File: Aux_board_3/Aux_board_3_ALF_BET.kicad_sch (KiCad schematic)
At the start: 37 parts, among them Q10 BSS84KJ, Q11 BSS138KJ, Q12 BSS84KJ, Q13 BSS138KJ, Q14 BSS84KJ, Q15 BSS138KJ, Q16 BSS84KJ, Q7 BSS138KJ, Q8 BSS84KJ, Q9 BSS138KJ

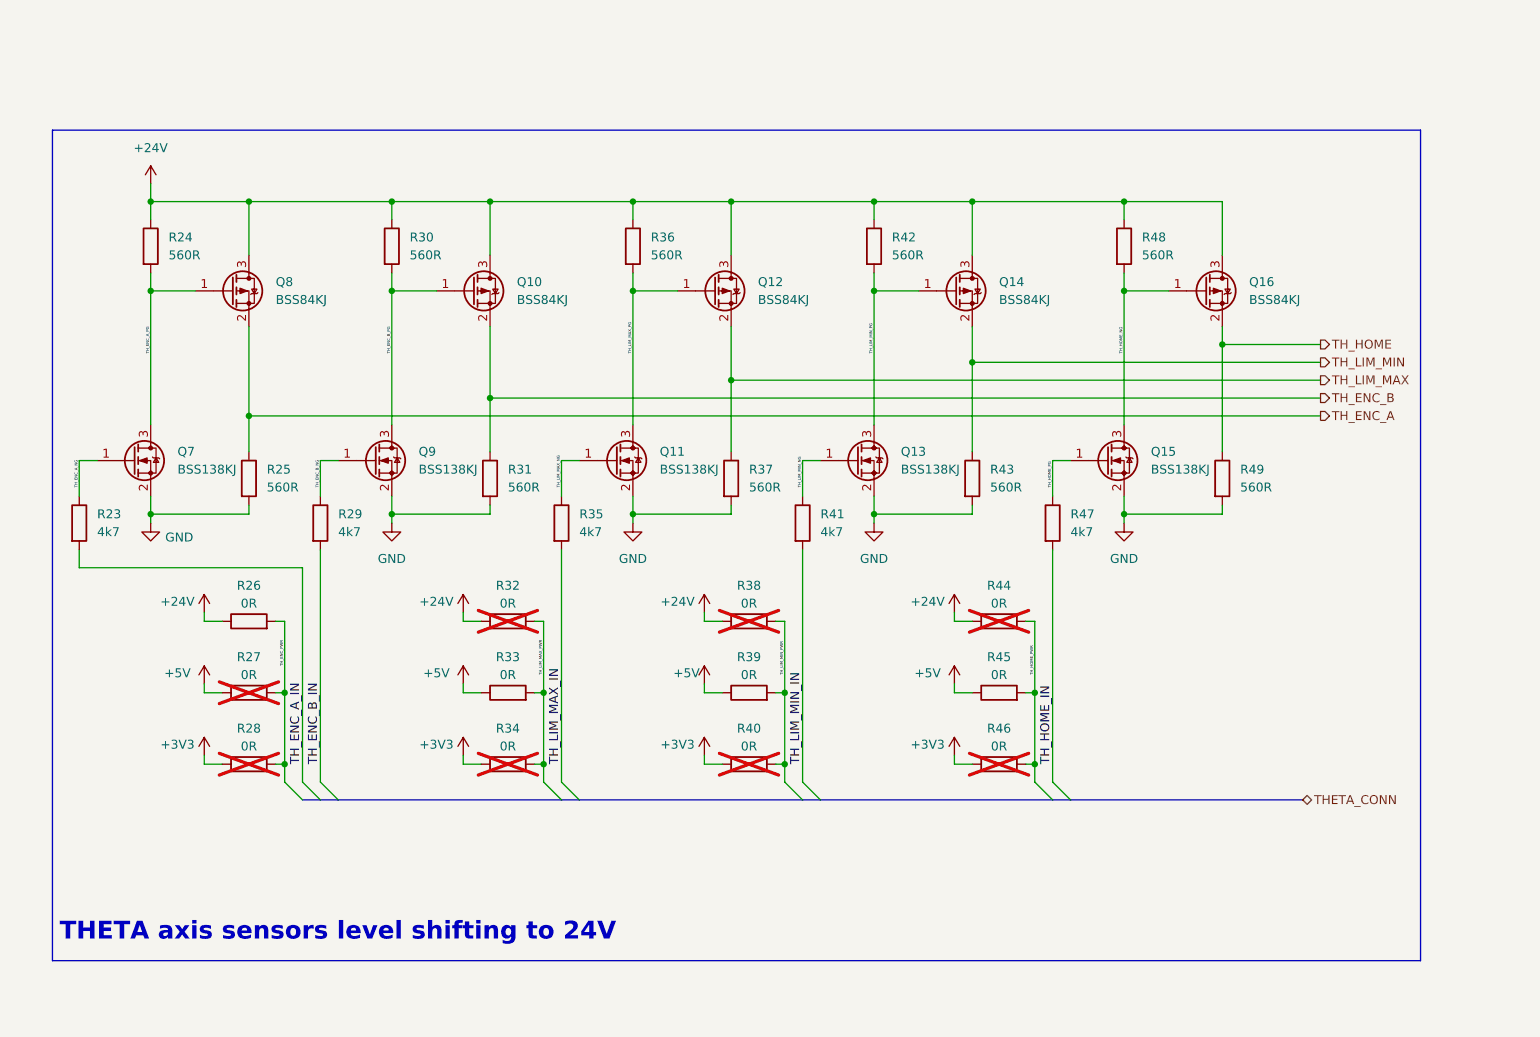
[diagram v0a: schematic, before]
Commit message: finished Board 3 schematic
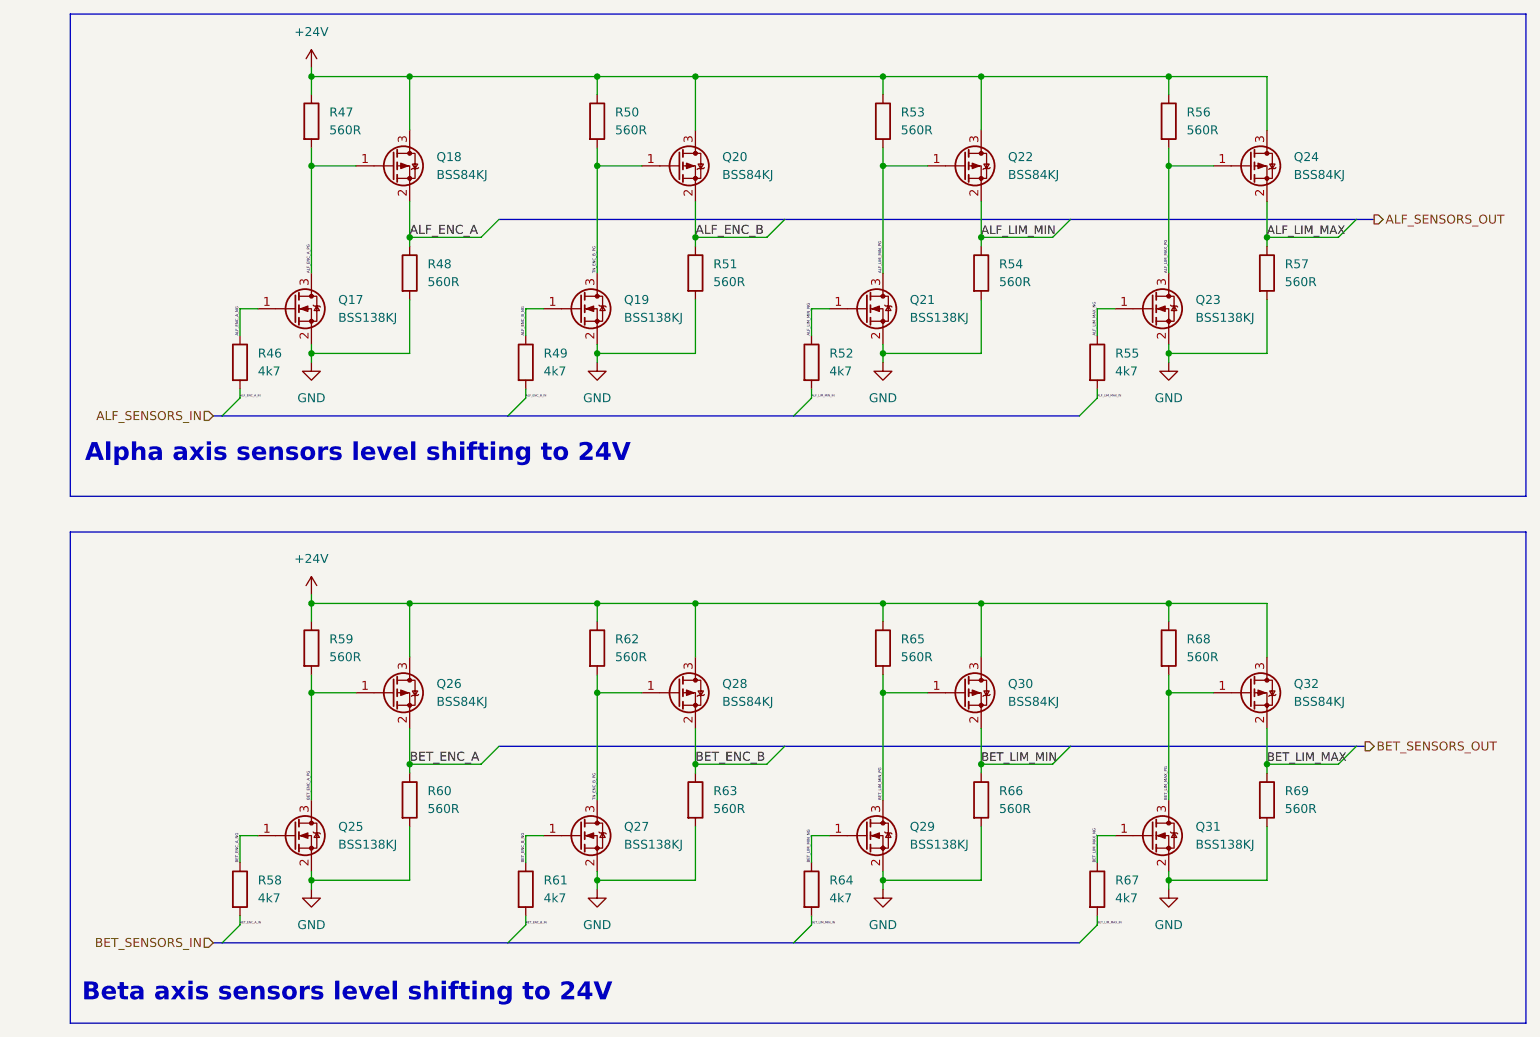
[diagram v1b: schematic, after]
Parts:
- removed Q10, Q12, Q14, Q16, Q8: BSS84KJ, Package_TO_SOT_SMD:SOT-23, symbol Transistor_FET:BSS84
- removed Q11, Q13, Q15, Q7, Q9: BSS138KJ, Package_TO_SOT_SMD:SOT-23, symbol Transistor_FET:BSS138
- removed R23, R29, R35, R41: 4k7, Resistor_SMD:R_0805_2012Metric_Pad1.20x1.40mm_HandSolder, symbol Device:R
- removed R24, R25, R30, R31, R36, R37, R42, R43: 560R, Resistor_SMD:R_0805_2012Metric_Pad1.20x1.40mm_HandSolder, symbol Device:R
- removed R26, R27, R28, R32, R33, R34, R38, R39, R40, R44, R45: 0R, Resistor_SMD:R_0805_2012Metric_Pad1.20x1.40mm_HandSolder, symbol Device:R
- added Q17, Q19, Q21, Q23, Q25, Q27, Q29, Q31: BSS138KJ, Package_TO_SOT_SMD:SOT-23, symbol Transistor_FET:BSS138
- added Q18, Q20, Q22, Q24, Q26, Q28, Q30, Q32: BSS84KJ, Package_TO_SOT_SMD:SOT-23, symbol Transistor_FET:BSS84
- added R50, R51, R53, R54, R56, R57, R59, R60, R62, R63, R65, R66, R68, R69: 560R, Resistor_SMD:R_0805_2012Metric_Pad1.20x1.40mm_HandSolder, symbol Device:R
- added R52, R55, R58, R61, R64, R67: 4k7, Resistor_SMD:R_0805_2012Metric_Pad1.20x1.40mm_HandSolder, symbol Device:R
- R46: value 0R -> 4k7; Sourced 0 -> 1; Supplier LCSC -> Lomex; Supplier URL https://www.lcsc.com/product-detail/Chip-Resistor-Surface-M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 -> (none); Supplier item no C304192 -> 81-10-95; now fitted
- R47: value 4k7 -> 560R; Supplier item no 81-10-95 -> 81-10-84
- R49: value 560R -> 4k7; Supplier item no 81-10-84 -> 81-10-95
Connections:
- net TH_HOME_NG is gone; now on net GND: R48.2
- net TH_HOME_PG is gone; now on net +24V: R47.1
- net +24V: now also Q18.3 (D), Q20.3 (D), Q22.3 (D), Q24.3 (D), Q26.3 (D), Q28.3 (D), Q30.3 (D), Q32.3 (D), R50.1, R53.1, R56.1, R59.1, R62.1, R65.1, R68.1; no longer R48.1
- net GND: now also Q17.2 (S), Q19.2 (S), Q21.2 (S), Q23.2 (S), Q25.2 (S), Q27.2 (S), Q29.2 (S), Q31.2 (S), R51.2, R54.2, R57.2, R60.2, R63.2, R66.2, R69.2; no longer R49.2
- net +3V3 renamed ALF_ENC_A_NG
- net ALF_ENC_A_NG: now also Q17.1 (G)
- net TH_HOME renamed ALF_ENC_B_NG
- net ALF_ENC_B_NG: now also Q19.1 (G)
- net TH_HOME_IN renamed ALF_ENC_A_PG
- net ALF_ENC_A_PG: now also Q17.3 (D), Q18.1 (G)
- net TH_HOME_PWR renamed ALF_ENC_A_IN
- new net ALF_ENC_A: Q18.2 (S), R48.1
- new net ALF_ENC_B: Q20.2 (S), R51.1
- new net ALF_ENC_B_IN: R49.2
- new net ALF_LIM_MAX: Q24.2 (S), R57.1
- new net ALF_LIM_MAX_IN: R55.2
- new net ALF_LIM_MAX_NG: Q23.1 (G), R55.1
- new net ALF_LIM_MAX_PG: Q23.3 (D), Q24.1 (G), R56.2
- new net ALF_LIM_MIN: Q22.2 (S), R54.1
- new net ALF_LIM_MIN_IN: R52.2
- new net ALF_LIM_MIN_NG: Q21.1 (G), R52.1
- new net ALF_LIM_MIN_PG: Q21.3 (D), Q22.1 (G), R53.2
- new net BET_ENC_A: Q26.2 (S), R60.1
- new net BET_ENC_A_IN: R58.2
- new net BET_ENC_A_NG: Q25.1 (G), R58.1
- new net BET_ENC_A_PG: Q25.3 (D), Q26.1 (G), R59.2
- new net BET_ENC_B: Q28.2 (S), R63.1
- new net BET_ENC_B_IN: R61.2
- new net BET_ENC_B_NG: Q27.1 (G), R61.1
- new net BET_LIM_MAX: Q32.2 (S), R69.1
- new net BET_LIM_MAX_IN: R67.2
- new net BET_LIM_MAX_NG: Q31.1 (G), R67.1
- new net BET_LIM_MAX_PG: Q31.3 (D), Q32.1 (G), R68.2
- new net BET_LIM_MIN: Q30.2 (S), R66.1
- new net BET_LIM_MIN_IN: R64.2
- new net BET_LIM_MIN_NG: Q29.1 (G), R64.1
- new net BET_LIM_MIN_PG: Q29.3 (D), Q30.1 (G), R65.2
- new net TN_ENC_B_PG: Q19.3 (D), Q20.1 (G), Q27.3 (D), Q28.1 (G), R50.2, R62.2
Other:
- note added: "Alpha axis sensors level shifting to 24V"
- note added: "Beta axis sensors level shifting to 24V"
- note removed: "THETA axis sensors level shifting to 24V"
